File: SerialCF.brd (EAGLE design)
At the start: 106.7 x 50.5 mm, 18 parts, among them IC1 XR-16C550P, T1 BC547, T2 BC547

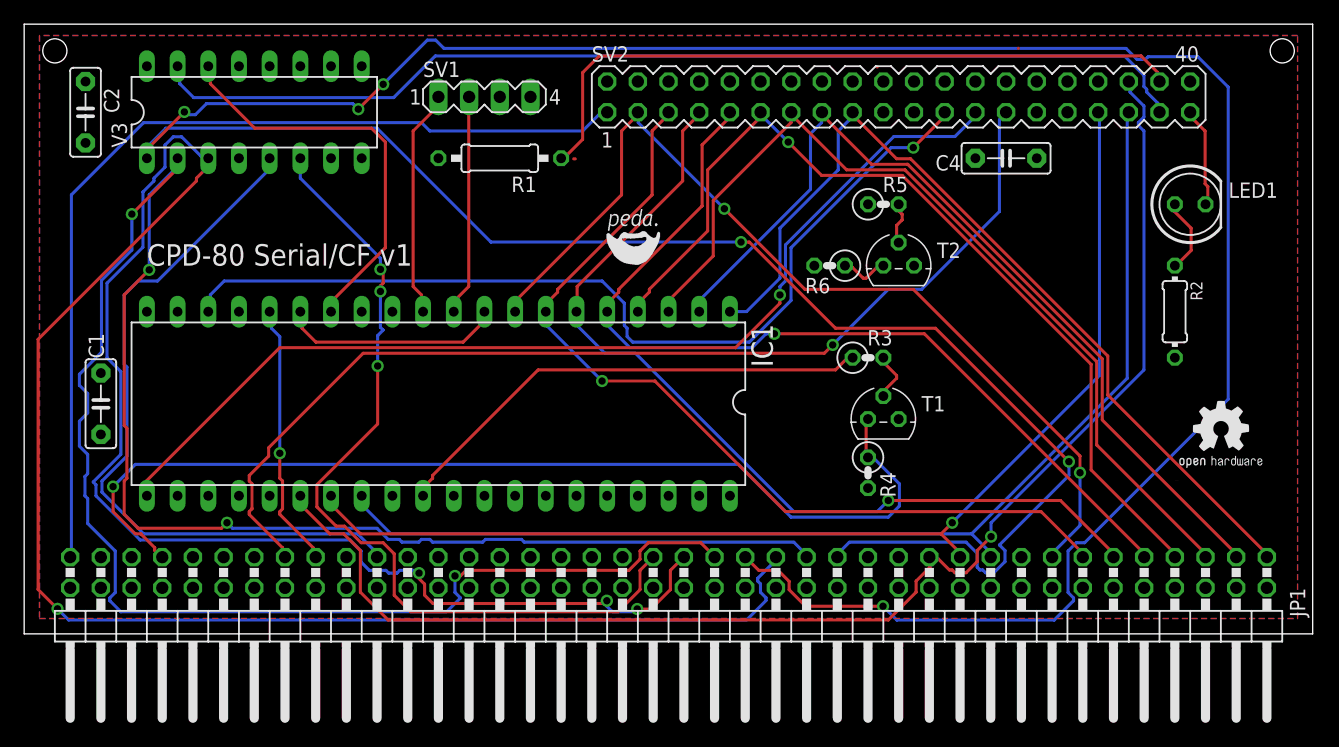
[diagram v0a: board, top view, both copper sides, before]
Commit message: Use LS version for serialCF
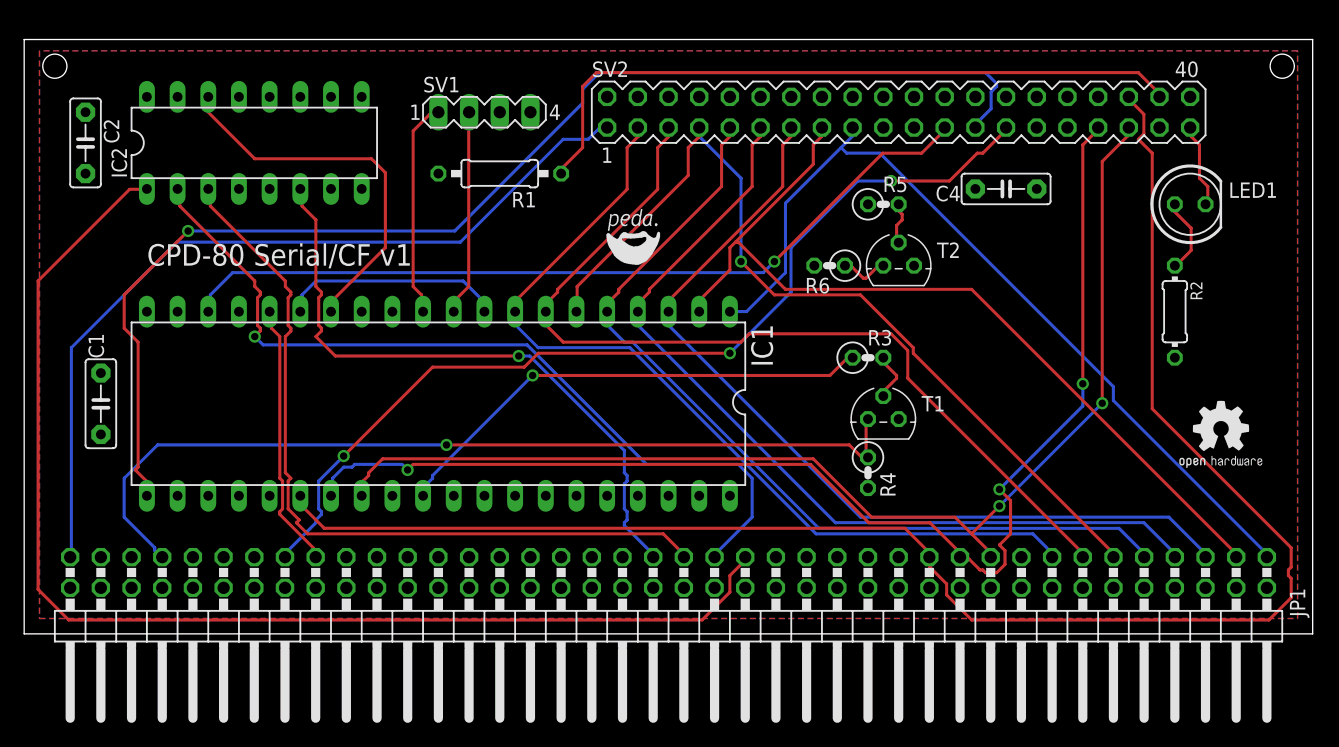
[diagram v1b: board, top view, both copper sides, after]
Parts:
- removed V3: 74138N, 74ttl-din:DIL16
- added IC2: 74LS138N, 74xx-eu:DIL16
- moved C2 2.54 mm to (5.08, 40.6)
- moved C4 2.54 mm to (81.3, 36.8)
- moved SV1 1.27 mm to (38.1, 43.2)
- moved SV2 1.27 mm to (72.4, 43.2)
- moved R1 1.27 mm to (39.4, 38.1)
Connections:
- net A10: now also IC2.3; no longer V3.3
- net A11: now also IC2.6; no longer V3.6
- net A8: now also IC2.1; no longer V3.1
- net A9: now also IC2.2; no longer V3.2
- net GND: now also IC2.8; no longer V3.4, V3.8
- net IOCS1: no longer V3.15
- net N$4: now also IC2.14; no longer V3.14
- net N$5: no longer V3.5
- net VCC: now also IC2.16; no longer V3.16
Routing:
- net A5: track 116.7 -> 0.00 mm, vias 2 -> 0
- net A7: track 108.0 -> 0.00 mm, vias 1 -> 0
- net A6: track 90.3 -> 0.00 mm, vias 2 -> 0
- net IOCS1: track 87.6 -> 0.00 mm
- net A8: track 175.3 -> 100.5 mm, vias 4 -> 0
- net N$5: track 59.7 -> 0.00 mm
- net A10: track 94.6 -> 65.2 mm, vias 3 -> 0
- net A9: track 97.7 -> 69.5 mm, vias 2 -> 1
- net A2: track 113.1 -> 136.3 mm, vias 1 -> 0
- net !RD: track 85.4 -> 102.9 mm
- net A11: track 70.6 -> 53.2 mm, vias 3 -> 1
- net N$9: track 84.6 -> 74.2 mm
- net WAIT: track 88.2 -> 79.1 mm, vias 1 -> 3
- net !WR: track 77.2 -> 68.4 mm
- net !RESET: track 77.8 -> 69.3 mm
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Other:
- board size 106.7 x 50.5 mm -> 106.7 x 49.2 mm

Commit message: Update SerialCF
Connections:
- net A11: now also IC2.4; no longer IC2.6
- net GND: now also IC2.6
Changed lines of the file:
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@@
 <contactref element="JP1" pad="80"/>
 <contactref element="IC2" pad="8"/>
+<contactref element="IC2" pad="6"/>
+<wire x1="83.82" y1="44.45" x2="96.52" y2="44.45" width="0" layer="19" extent="1-1"/>
+<wire x1="78.74" y1="44.45" x2="83.82" y2="44.45" width="0" layer="19" extent="1-1"/>
+<wire x1="76.2" y1="44.45" x2="78.74" y2="44.45" width="0" layer="19" extent="1-1"/>
+<wire x1="73.66" y1="44.45" x2="76.2" y2="44.45" width="0" layer="19" extent="1-1"/>
+<wire x1="71.12" y1="41.91" x2="73.66" y2="44.45" width="0" layer="19" extent="1-1"/>
+<wire x1="83.82" y1="36.83" x2="83.82" y2="44.45" width="0" layer="19" extent="1-1"/>
+<wire x1="73.66" y1="30.48" x2="71.12" y2="41.91" width="0" layer="19" extent="1-1"/>
+<wire x1="72.39" y1="17.78" x2="73.66" y2="30.48" width="0" layer="19" extent="1-1"/>
+<wire x1="72.39" y1="3.81" x2="72.39" y2="17.78" width="0" layer="19" extent="1-1"/>
+<wire x1="74.93" y1="3.81" x2="72.39" y2="3.81" width="0" layer="19" extent="1-1"/>
+<wire x1="77.47" y1="3.81" x2="74.93" y2="3.81" width="0" layer="19" extent="1-1"/>
+<wire x1="80.01" y1="3.81" x2="77.47" y2="3.81" width="0" layer="19" extent="1-1"/>
+<wire x1="82.55" y1="3.81" x2="80.01" y2="3.81" width="0" layer="19" extent="1-1"/>
+<wire x1="82.55" y1="6.35" x2="82.55" y2="3.81" width="0" layer="19" extent="1-1"/>
+<wire x1="85.09" y1="3.81" x2="82.55" y2="3.81" width="0" layer="19" extent="1-1"/>
+<wire x1="87.63" y1="3.81" x2="85.09" y2="3.81" width="0" layer="19" extent="1-1"/>
+<wire x1="90.17" y1="3.81" x2="87.63" y2="3.81" width="0" layer="19" extent="1-1"/>
+<wire x1="92.71" y1="3.81" x2="90.17" y2="3.81" width="0" layer="19" extent="1-1"/>
+<wire x1="95.25" y1="3.81" x2="92.71" y2="3.81" width="0" layer="19" extent="1-1"/>
+<wire x1="97.79" y1="3.81" x2="95.25" y2="3.81" width="0" layer="19" extent="1-1"/>
+<wire x1="100.33" y1="3.81" x2="97.79" y2="3.81" width="0" layer="19" extent="1-1"/>
+<wire x1="102.87" y1="3.81" x2="100.33" y2="3.81" width="0" layer="19" extent="1-1"/>
+<wire x1="69.85" y1="3.81" x2="72.39" y2="3.81" width="0" layer="19" extent="1-1"/>
+<wire x1="67.31" y1="3.81" x2="69.85" y2="3.81" width="0" layer="19" extent="1-1"/>
+<wire x1="64.77" y1="3.81" x2="67.31" y2="3.81" width="0" layer="19" extent="1-1"/>
+<wire x1="62.23" y1="3.81" x2="64.77" y2="3.81" width="0" layer="19" extent="1-1"/>
+<wire x1="59.69" y1="3.81" x2="62.23" y2="3.81" width="0" layer="19" extent="1-1"/>
+<wire x1="57.15" y1="3.81" x2="59.69" y2="3.81" width="0" layer="19" extent="1-1"/>
+<wire x1="54.61" y1="3.81" x2="57.15" y2="3.81" width="0" layer="19" extent="1-1"/>
+<wire x1="52.07" y1="3.81" x2="54.61" y2="3.81" width="0" layer="19" extent="1-1"/>
+<wire x1="49.53" y1="3.81" x2="52.07" y2="3.81" width="0" layer="19" extent="1-1"/>
+<wire x1="46.99" y1="3.81" x2="49.53" y2="3.81" width="0" layer="19" extent="1-1"/>
+<wire x1="44.45" y1="3.81" x2="46.99" y2="3.81" width="0" layer="19" extent="1-1"/>
+<wire x1="41.91" y1="3.81" x2="44.45" y2="3.81" width="0" layer="19" extent="1-1"/>
+<wire x1="39.37" y1="3.81" x2="41.91" y2="3.81" width="0" layer="19" extent="1-1"/>
+<wire x1="39.37" y1="6.35" x2="39.37" y2="3.81" width="0" layer="19" extent="1-1"/>
+<wire x1="36.83" y1="3.81" x2="39.37" y2="3.81" width="0" layer="19" extent="1-1"/>
+<wire x1="34.29" y1="3.81" x2="36.83" y2="3.81" width="0" layer="19" extent="1-1"/>
+<wire x1="31.75" y1="3.81" x2="34.29" y2="3.81" width="0" layer="19" extent="1-1"/>
+<wire x1="29.21" y1="3.81" x2="31.75" y2="3.81" width="0" layer="19" extent="1-1"/>
+<wire x1="26.67" y1="3.81" x2="29.21" y2="3.81" width="0" layer="19" extent="1-1"/>
+<wire x1="24.13" y1="3.81" x2="26.67" y2="3.81" width="0" layer="19" extent="1-1"/>
+<wire x1="21.59" y1="3.81" x2="24.13" y2="3.81" width="0" layer="19" extent="1-1"/>
+<wire x1="19.05" y1="3.81" x2="21.59" y2="3.81" width="0" layer="19" extent="1-1"/>
+<wire x1="16.51" y1="3.81" x2="19.05" y2="3.81" width="0" layer="19" extent="1-1"/>
+<wire x1="13.97" y1="3.81" x2="16.51" y2="3.81" width="0" layer="19" extent="1-1"/>
+<wire x1="11.43" y1="3.81" x2="13.97" y2="3.81" width="0" layer="19" extent="1-1"/>
+<wire x1="8.89" y1="3.81" x2="11.43" y2="3.81" width="0" layer="19" extent="1-1"/>
+<wire x1="6.35" y1="3.81" x2="8.89" y2="3.81" width="0" layer="19" extent="1-1"/>
+<wire x1="3.81" y1="3.81" x2="6.35" y2="3.81" width="0" layer="19" extent="1-1"/>
+<wire x1="20.32" y1="11.43" x2="21.59" y2="3.81" width="0" layer="19" extent="1-1"/>
+<wire x1="12.7" y1="11.43" x2="20.32" y2="11.43" width="0" layer="19" extent="1-1"/>
+<wire x1="6.35" y1="16.51" x2="12.7" y2="11.43" width="0" layer="19" extent="1-1"/>
+<wire x1="10.16" y1="26.67" x2="6.35" y2="16.51" width="0" layer="19" extent="1-1"/>
+<wire x1="12.7" y1="26.67" x2="10.16" y2="26.67" width="0" layer="19" extent="1-1"/>
+<wire x1="5.08" y1="38.1" x2="10.16" y2="26.67" width="0" layer="19" extent="1-1"/>
+<wire x1="22.86" y1="36.83" x2="12.7" y2="26.67" width="0" layer="19" extent="1-1"/>
+<wire x1="27.94" y1="36.83" x2="22.86" y2="36.83" width="0" layer="19" extent="1-1"/>
+<wire x1="41.91" y1="43.18" x2="27.94" y2="36.83" width="0" layer="19" extent="1-1"/>
+<wire x1="48.26" y1="44.45" x2="41.91" y2="43.18" width="0" layer="19" extent="1-1"/>
 </signal>
 <signal name="A0">
@@
 <signal name="A11">
 <contactref element="JP1" pad="41"/>
-<contactref element="IC2" pad="6"/>
 <wire x1="23" y1="35.42" x2="23" y2="36.8" width="0.254" layer="1"/>
 <wire x1="24.15" y1="34.27" x2="23" y2="35.42" width="0.254" layer="1"/>
@@
 <wire x1="49.68" y1="8.97" x2="49.68" y2="9.2" width="0.254" layer="16"/>
 <wire x1="52.21" y1="6.44" x2="49.68" y2="8.97" width="0.254" layer="16"/>
-<wire x1="23" y1="36.8" x2="22.86" y2="36.83" width="0.254" layer="1"/>
 <wire x1="52.21" y1="6.44" x2="52.07" y2="6.35" width="0.254" layer="16"/>
 <via x="40.94" y="23" extent="1-16" drill="0.6096"/>
+<contactref element="IC2" pad="4"/>
+<wire x1="23" y1="36.8" x2="17.78" y2="36.83" width="0" layer="19" extent="1-1"/>
 </signal>
 <signal name="A12">
